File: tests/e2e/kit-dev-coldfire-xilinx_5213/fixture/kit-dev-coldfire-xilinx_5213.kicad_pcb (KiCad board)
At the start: 4 copper layers, 157.5 x 91.4 mm, 160 parts, among them J201 JACK_2P, P301 CONN_6, P302 CONN_2X2, P303 CONN_20X2, Q101 3906, SW201 SW_PUSH, SW202 SW_PUSH, U101 74AHC1G14, U102 MCF5213-LQFP100, U201 74HC125, U202 MAX202, U203 MAX202, U204 MAX202, U205 PCA82C251, U301 XCR3256-TQ144, Y101 8MHz

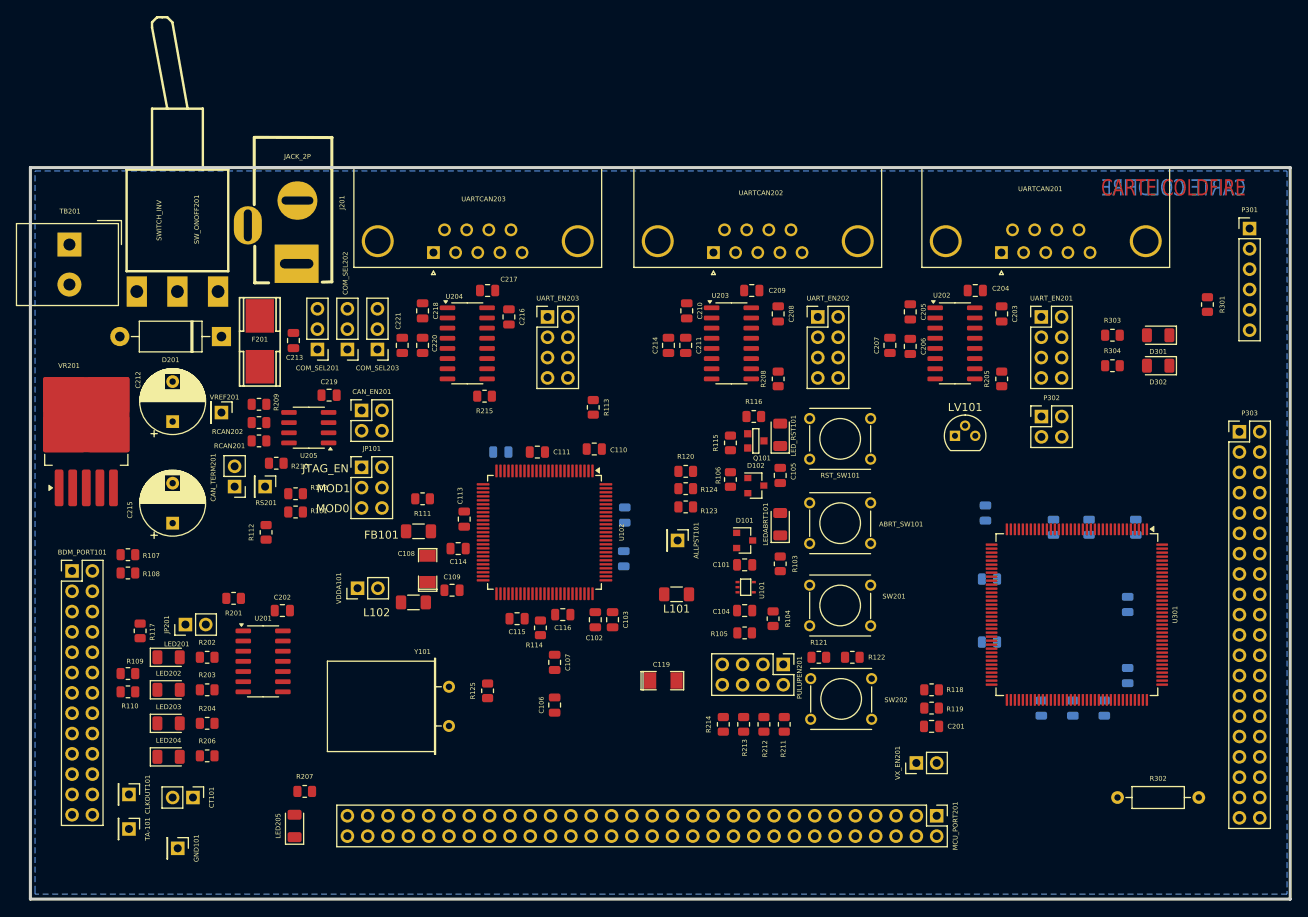
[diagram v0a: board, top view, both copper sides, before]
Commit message: e2e
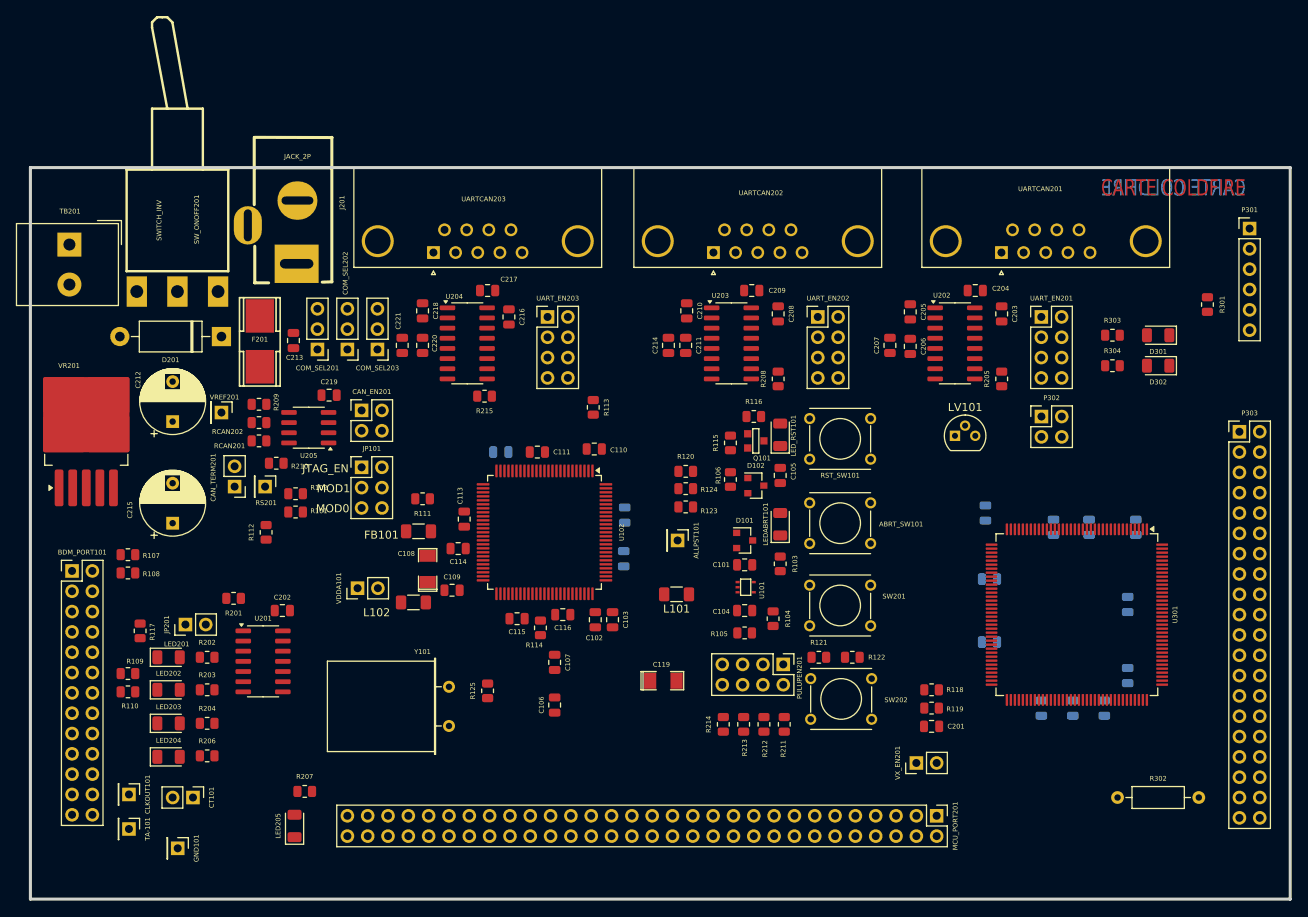
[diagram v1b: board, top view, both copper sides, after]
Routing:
- removed copper zone on In2.Cu, net +3.3V
- removed copper zone on B.Cu, net GND
- removed copper zone on In1.Cu, net GND
